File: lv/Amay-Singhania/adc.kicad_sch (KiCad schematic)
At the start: 2 parts, among them J1 Conn_01x07_Pin, U4 ADS127L01xPBS

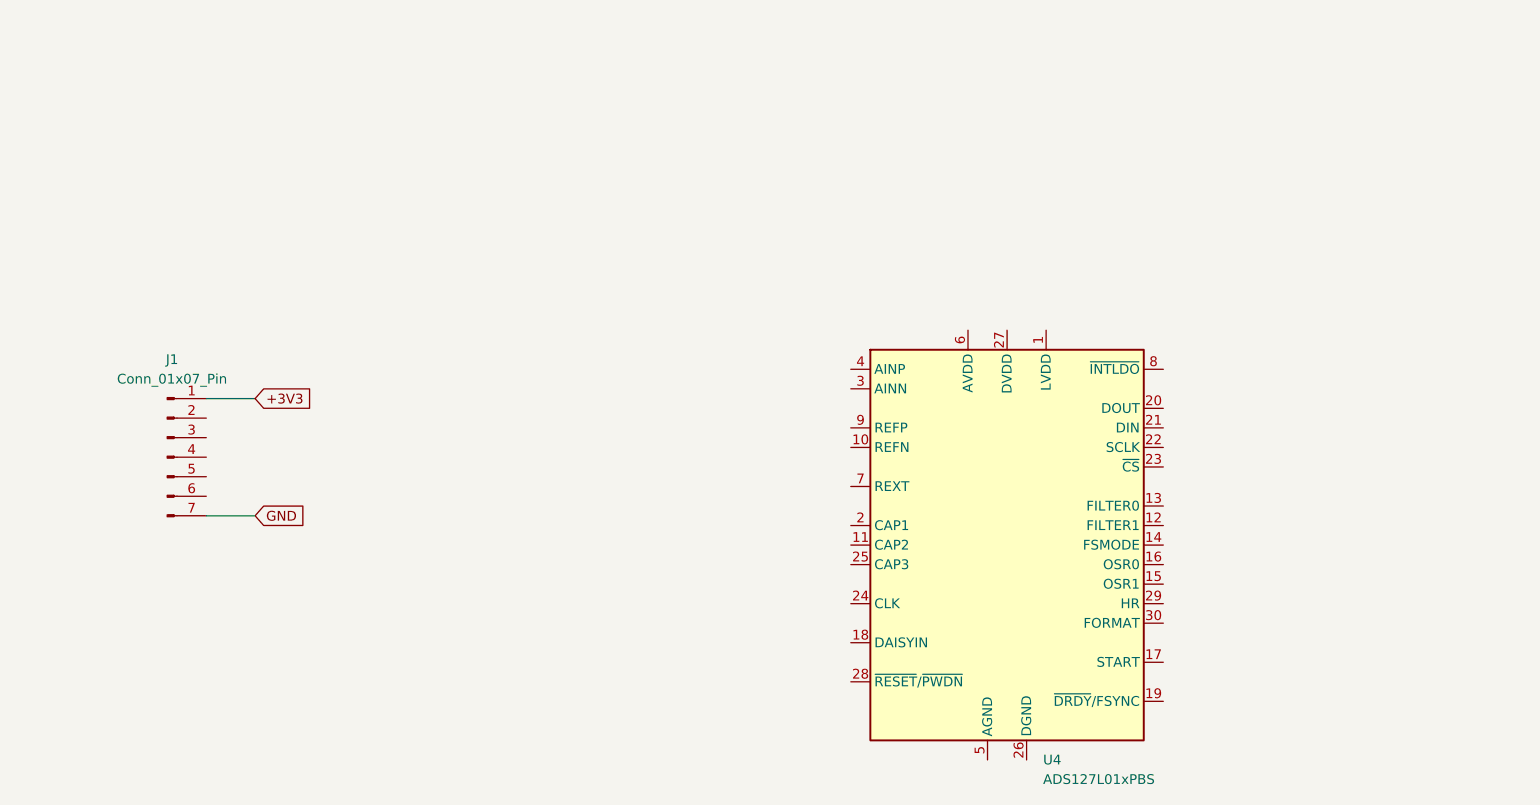
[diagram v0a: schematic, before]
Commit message: lv and fw changes
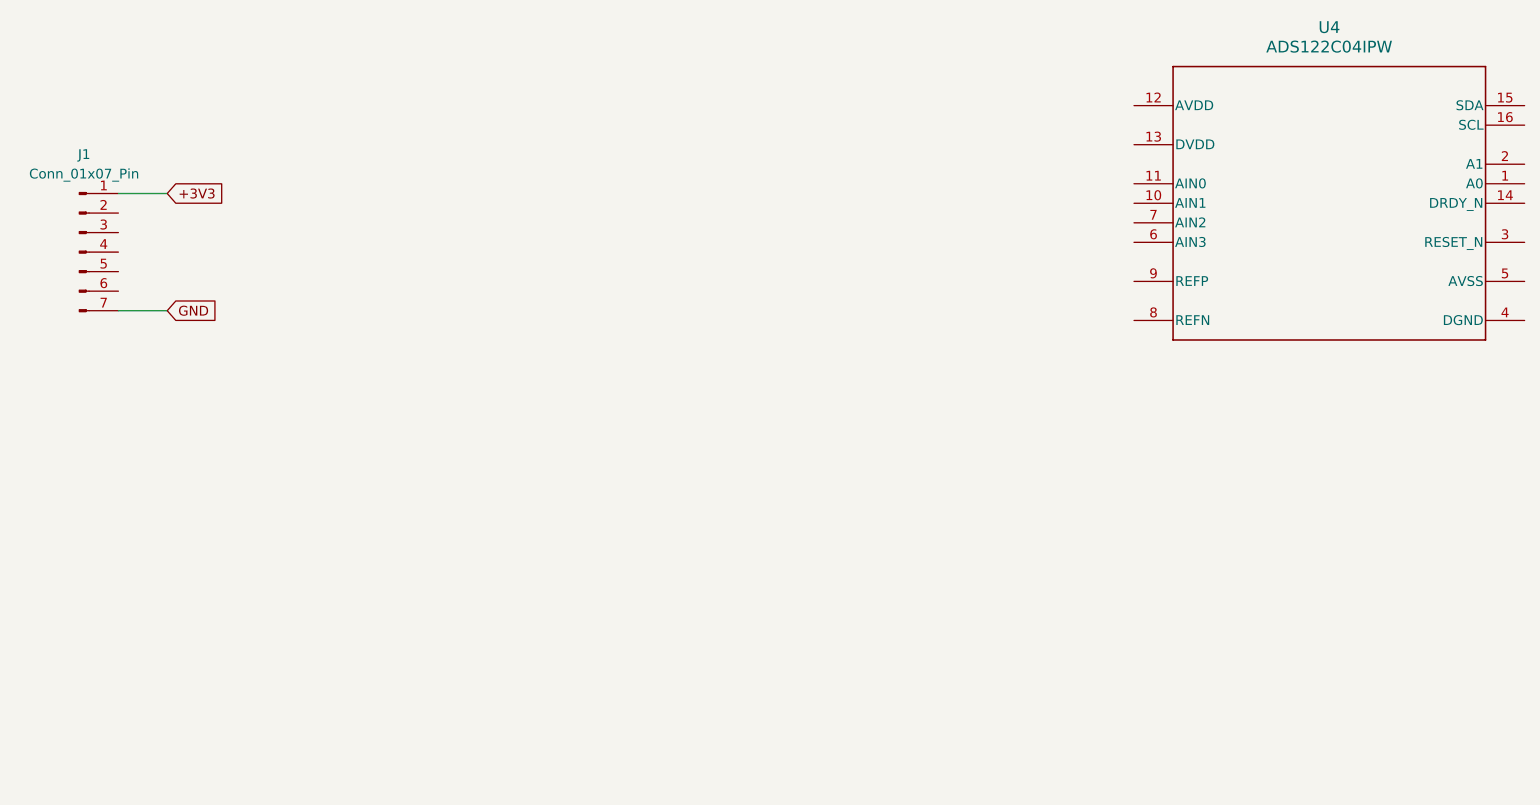
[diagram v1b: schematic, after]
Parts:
- removed U4: ADS127L01xPBS, ADS127L01xPBS:VQFN56_RSH_TEX, symbol Analog_ADC:ADS127L01xPBS
- added U4: ADS122C04IPW, PW0016A_N, symbol ADS122C04:ADS122C04IPW
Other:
- moved on the sheet: J1
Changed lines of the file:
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@@
 	(wire
 		(pts
-			(xy 49.53 78.74) (xy 55.88 78.74)
+			(xy 38.1 52.07) (xy 44.45 52.07)
 		)
 		(stroke
@@
 	(wire
 		(pts
-			(xy 49.53 93.98) (xy 55.88 93.98)
+			(xy 38.1 67.31) (xy 44.45 67.31)
 		)
 		(stroke
@@
 	(global_label "+3V3"
 		(shape input)
-		(at 55.88 78.74 0)
+		(at 44.45 52.07 0)
 		(fields_autoplaced yes)
 		(effects
@@
 		)
 		(property "Intersheetrefs" "${INTERSHEET_REFS}"
-			(at 63.9452 78.74 0)
+			(at 52.5152 52.07 0)
 			(hide yes)
 			(show_name no)
@@
 	(global_label "GND"
 		(shape input)
-		(at 55.88 93.98 0)
+		(at 44.45 67.31 0)
 		(fields_autoplaced yes)
 		(effects
@@
 		)
 		(property "Intersheetrefs" "${INTERSHEET_REFS}"
-			(at 62.7357 93.98 0)
+			(at 51.3057 67.31 0)
 			(hide yes)
 			(show_name no)
@@
 	)
 	(symbol
-		(lib_id "Analog_ADC:ADS127L01xPBS")
-		(at 153.67 97.79 0)
+		(lib_id "ADS122C04:ADS122C04IPW")
+		(at 195.58 53.34 0)
 		(unit 1)
 		(body_style 1)
@@
 		(fields_autoplaced yes)
 		(property "Reference" "U4"
-			(at 158.3533 125.73 0)
-			(show_name no)
-			(do_not_autoplace no)
-			(effects
-				(font
-					(size 1.27 1.27)
-				)
-				(justify left)
-			)
-		)
-		(property "Value" "ADS127L01xPBS"
-			(at 158.3533 128.27 0)
-			(show_name no)
-			(do_not_autoplace no)
-			(effects
-				(font
-					(size 1.27 1.27)
-				)
-				(justify left)
-			)
-		)
-		(property "Footprint" "ADS127L01xPBS:VQFN56_RSH_TEX"
-			(at 153.67 97.79 0)
-			(hide yes)
-			(show_name no)
-			(do_not_autoplace no)
-			(effects
-				(font
-					(size 1.27 1.27)
-				)
-			)
-		)
-		(property "Datasheet" "https://www.ti.com/lit/ds/symlink/ads127l01.pdf"
-			(at 153.67 97.79 0)
-			(hide yes)
-			(show_name no)
-			(do_not_autoplace no)
-			(effects
-				(font
-					(size 1.27 1.27)
-				)
-			)
-		)
-		(property "Description" "24-bit delta-sigma ADC, Single Channel, 512 kSPS, SPI & Frame-Sync interface, TQFP-32"
-			(at 153.67 97.79 0)
-			(hide yes)
-			(show_name no)
-			(do_not_autoplace no)
-			(effects
-				(font
-					(size 1.27 1.27)
-				)
-			)
-		)
-		(property "Digikey Part Number" ""
-			(at 153.67 97.79 0)
-			(hide yes)
-			(show_name no)
-			(do_not_autoplace no)
-			(effects
-				(font
-					(size 1.27 1.27)
-				)
-			)
-		)
-		(property "Digikey URL" ""
-			(at 153.67 97.79 0)
-			(hide yes)
-			(show_name no)
-			(do_not_autoplace no)
-			(effects
-				(font
-					(size 1.27 1.27)
-				)
-			)
-		)
-		(property "Manufacturer" ""
-			(at 153.67 97.79 0)
-			(hide yes)
-			(show_name no)
-			(do_not_autoplace no)
-			(effects
-				(font
-					(size 1.27 1.27)
-				)
-			)
-		)
-		(property "Manufacturer Part Number" ""
-			(at 153.67 97.79 0)
-			(hide yes)
-			(show_name no)
-			(do_not_autoplace no)
-			(effects
-				(font
-					(size 1.27 1.27)
-				)
-			)
-		)
-		(pin "22"
-		)
-		(pin "20"
-		)
-		(pin "21"
-		)
-		(pin "17"
-		)
-		(pin "19"
-		)
-		(pin "18"
-		)
-		(pin "31"
+			(at 195.58 30.48 0)
+			(show_name no)
+			(do_not_autoplace no)
+			(effects
+				(font
+					(size 1.524 1.524)
+				)
+			)
+		)
+		(property "Value" "ADS122C04IPW"
+			(at 195.58 33.02 0)
+			(show_name no)
+			(do_not_autoplace no)
+			(effects
+				(font
+					(size 1.524 1.524)
+				)
+			)
+		)
+		(property "Footprint" "PW0016A_N"
+			(at 195.58 53.34 0)
+			(hide yes)
+			(show_name no)
+			(do_not_autoplace no)
+			(effects
+				(font
+					(size 1.27 1.27)
+					(italic yes)
+				)
+			)
+		)
+		(property "Datasheet" "https://www.ti.com/lit/gpn/ads122c04"
+			(at 195.58 53.34 0)
+			(hide yes)
+			(show_name no)
+			(do_not_autoplace no)
+			(effects
+				(font
+					(size 1.27 1.27)
+					(italic yes)
+				)
+			)
+		)
+		(property "Description" ""
+			(at 195.58 53.34 0)
+			(hide yes)
+			(show_name no)
+			(do_not_autoplace no)
+			(effects
+				(font
+					(size 1.27 1.27)
+				)
+			)
+		)
+		(pin "16"
 		)
 		(pin "12"
 		)
+		(pin "11"
+		)
+		(pin "1"
+		)
+		(pin "4"
+		)
+		(pin "3"
+		)
+		(pin "5"
+		)
+		(pin "6"
+		)
+		(pin "13"
+		)
+		(pin "14"
+		)
+		(pin "7"
+		)
+		(pin "8"
+		)
+		(pin "9"
+		)
+		(pin "10"
+		)
+		(pin "15"
+		)
 		(pin "2"
-		)
-		(pin "9"
-		)
-		(pin "11"
-		)
-		(pin "32"
-		)
-		(pin "3"
-		)
-		(pin "30"
-		)
-		(pin "23"
-		)
-		(pin "10"
-		)
-		(pin "4"
-		)
-		(pin "5"
-		)
-		(pin "8"
-		)
-		(pin "7"
-		)
-		(pin "26"
-		)
-		(pin "25"
-		)
-		(pin "24"
-		)
-		(pin "29"
-		)
-		(pin "13"
-		)
-		(pin "28"
-		)
-		(pin "1"
-		)
-		(pin "27"
-		)
-		(pin "14"
-		)
-		(pin "6"
-		)
-		(pin "15"
-		)
-		(pin "16"
 		)
 		(instances
@@
 	(symbol
 		(lib_id "Connector:Conn_01x07_Pin")
-		(at 44.45 86.36 0)
+		(at 33.02 59.69 0)
 		(unit 1)
 		(body_style 1)
@@
 		(fields_autoplaced yes)
 		(property "Reference" "J1"
-			(at 45.085 73.66 0)
+			(at 33.655 46.99 0)
 			(show_name no)
 			(do_not_autoplace no)
@@
 		)
 		(property "Value" "Conn_01x07_Pin"
-			(at 45.085 76.2 0)
+			(at 33.655 49.53 0)
 			(show_name no)
 			(do_not_autoplace no)
@@
 		)
 		(property "Footprint" "Connector_Harwin:Harwin_M20-89007xx_1x07_P2.54mm_Horizontal"
-			(at 44.45 86.36 0)
+			(at 33.02 59.69 0)
 			(hide yes)
 			(show_name no)
@@
 		)
 		(property "Datasheet" ""
-			(at 44.45 86.36 0)
+			(at 33.02 59.69 0)
 			(hide yes)
 			(show_name no)
@@
 		)
 		(property "Description" "Generic connector, single row, 01x07, script generated"
-			(at 44.45 86.36 0)
-			(hide yes)
-			(show_name no)
+			(at 33.02 59.69 0)
+			(hide yes)
+			(show_name no)
